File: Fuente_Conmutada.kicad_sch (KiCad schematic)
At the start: 50 parts, among them J1 Terminal_220v, J2 Terminal_12v, J3 Vout, Q1 IRF840, Q2 IRF840, T1 Transformer_1P_SS, U1 TL494, U2 IR2110

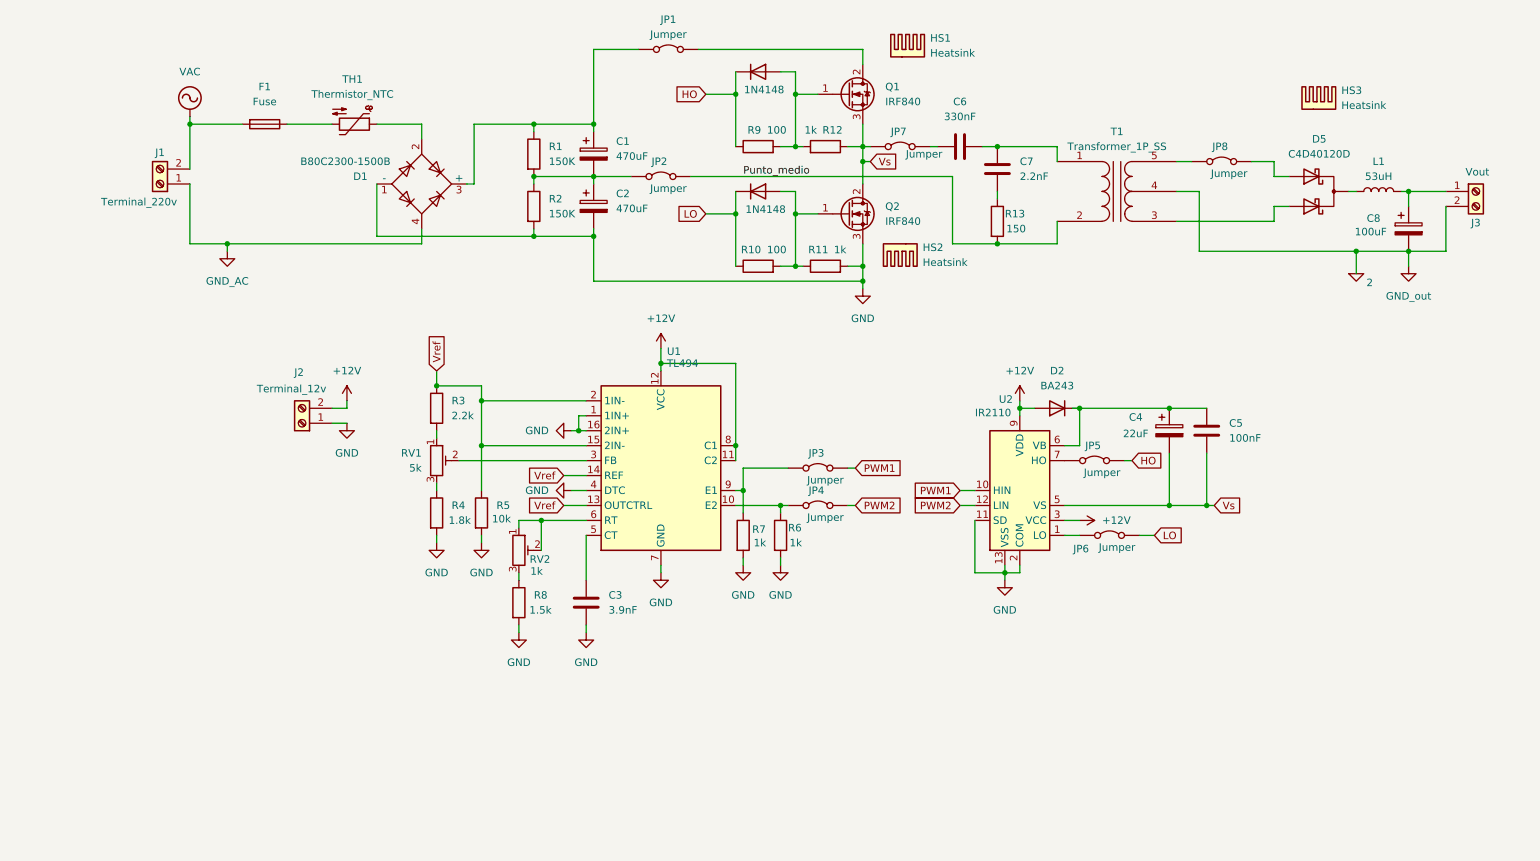
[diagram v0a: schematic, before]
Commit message: Esquemático
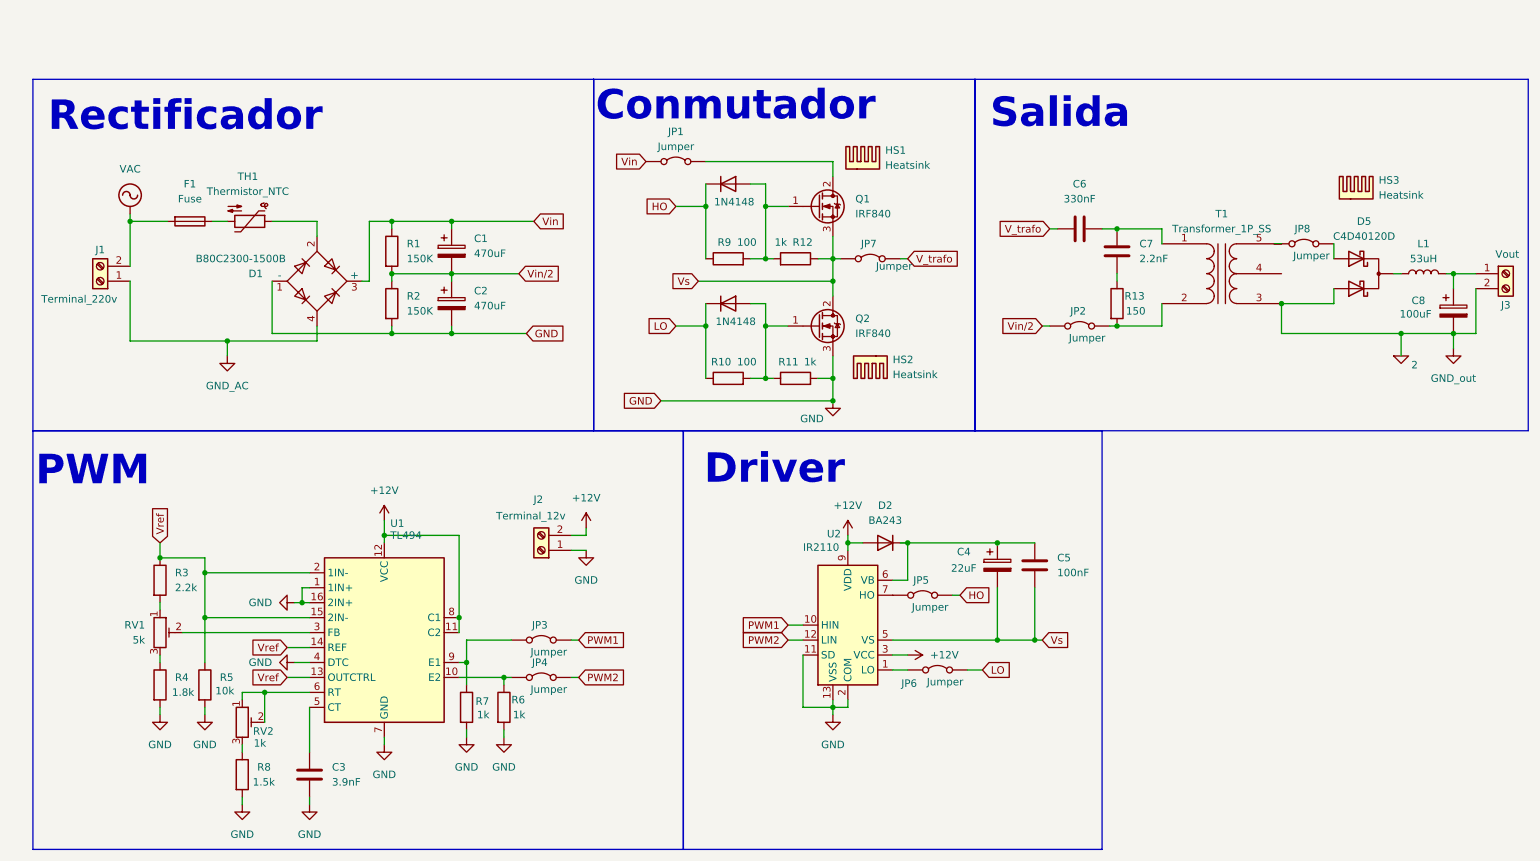
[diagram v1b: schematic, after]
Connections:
- net 2: now also D5.3 (A2), T1.3 (SA); no longer T1.4 (SC)
- net Vin/2: now reaches C1.2, C2.1, JP2.1 (A), R1.2, R2.1
- net Vin: now reaches C1.1, D1.3 (+), JP1.1 (A), R1.1
- net V_trafo: now reaches C6.2, JP7.2 (B)
- net Punto_medio: no longer names the net of JP2.2 (B), R13.2, T1.2 (AB)
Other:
- note added: "Conmutador"
- note added: "Driver"
- note added: "PWM"
- note added: "Rectificador"
- note added: "Salida"
- title: (none) -> Fuente Conmutada
- moved on the sheet: C1, C2, C3, C4, C5, C6, C7, C8, D1, D2, D5, F1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
